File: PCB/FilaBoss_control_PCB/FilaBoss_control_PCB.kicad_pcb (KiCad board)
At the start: 2 copper layers, 1 part, among them U1 WEMOS_C3_mini

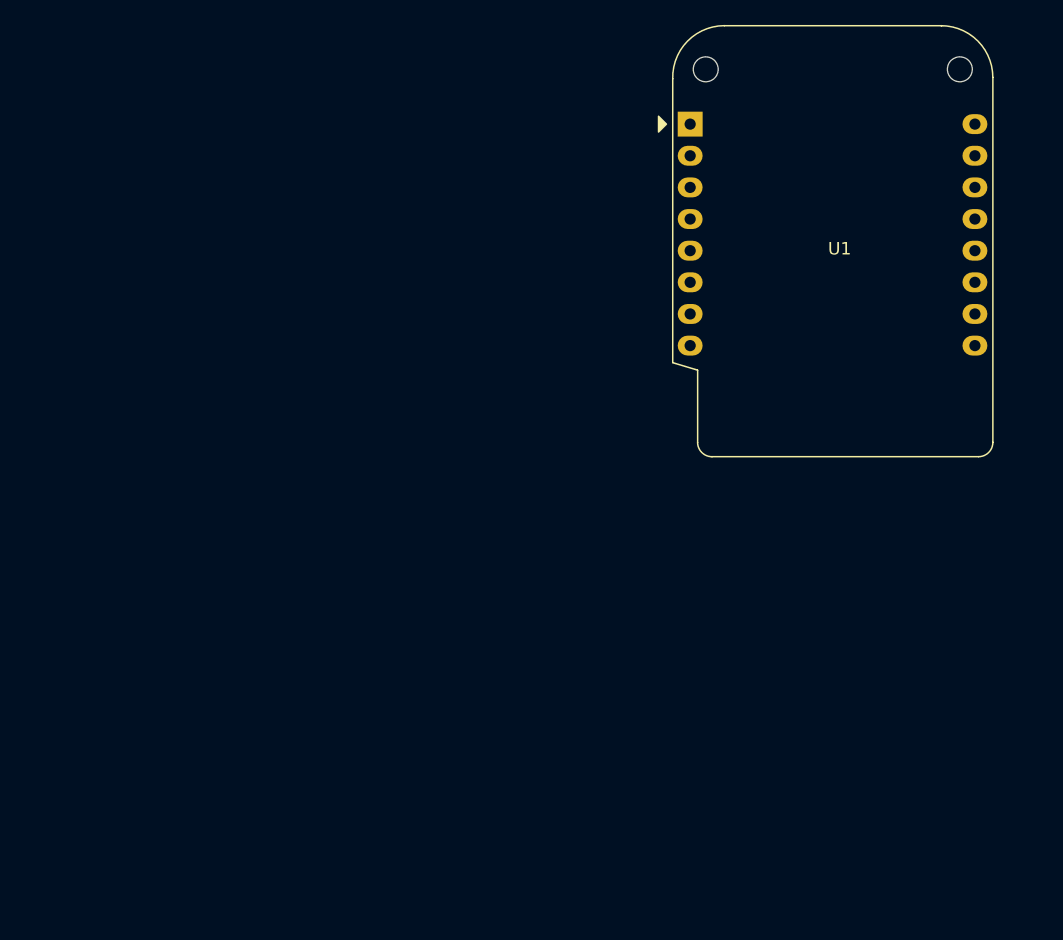
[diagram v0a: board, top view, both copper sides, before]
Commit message: pcb v1 ready
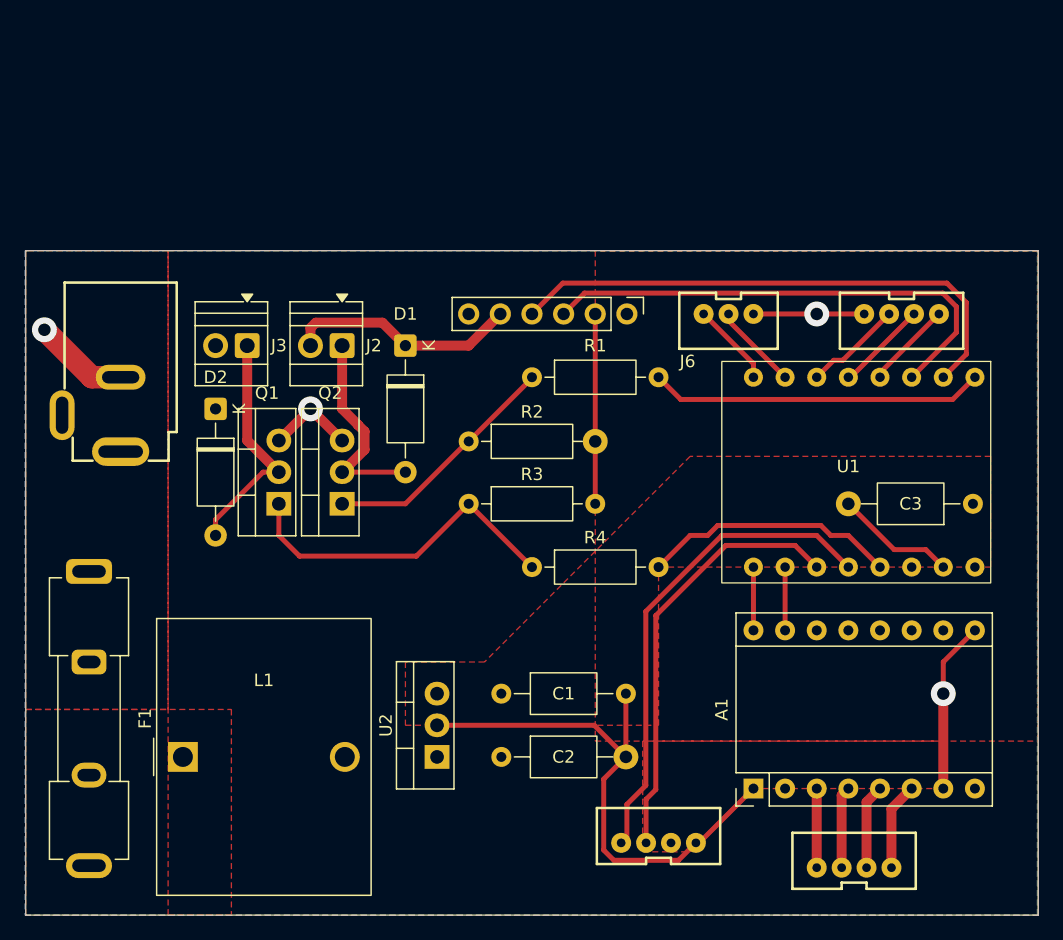
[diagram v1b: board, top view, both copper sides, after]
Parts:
- added A1: Pololu_Breakout_A4988, Module:Pololu_Breakout-16_15.2x20.3mm, F.Cu at (96.5, 129.5)
- added C1: C, Capacitor_THT:C_Axial_L5.1mm_D3.1mm_P10.00mm_Horizontal, F.Cu at (76.3, 121.9)
- added C2: C, Capacitor_THT:C_Axial_L5.1mm_D3.1mm_P10.00mm_Horizontal, F.Cu at (76.3, 127.0)
- added C3: C, Capacitor_THT:C_Axial_L5.1mm_D3.1mm_P10.00mm_Horizontal, F.Cu at (114.1, 106.7)
- added D1: D, Diode_THT:D_A-405_P10.16mm_Horizontal, F.Cu at (68.6, 94.0)
- added D2: D, Diode_THT:D_A-405_P10.16mm_Horizontal, F.Cu at (53.3, 99.1)
- added F1: Fuse, Fuse:Fuseholder_Clip-5x20mm_Keystone_3512P_Inline_P23.62x7.27mm_D1.02x2.41x1.02x1.57mm_Horizontal, F.Cu at (43.2, 112.1)
- added J1: Conn_01x04_Encoder, PCM_SparkFun-Connector:JST_1x04_P2.0mm_Vertical_PTH, F.Cu at (88.9, 133.3)
- added J2: Screw_Terminal_01x02, TerminalBlock:TerminalBlock_Xinya_XY308-2.54-2P_1x02_P2.54mm_Horizontal, F.Cu at (63.5, 94.0)
- added J3: Screw_Terminal_01x02, TerminalBlock:TerminalBlock_Xinya_XY308-2.54-2P_1x02_P2.54mm_Horizontal, F.Cu at (55.9, 94.0)
- added J5: Barrel_Jack_PTH_Slot, PCM_SparkFun-Connector:Barrel_Jack_PTH_Slot, F.Cu at (45.7, 96.5)
- added J6: PinHeader_01x06_P2.54mm_Vertical_THT_D1mm, PCM_fab:PinHeader_01x06_P2.54mm_Vertical_THT_D1mm, F.Cu at (86.4, 91.4)
- added J7: Conn_01x04, PCM_SparkFun-Connector:JST_1x04_P2.0mm_Vertical_PTH, F.Cu at (104.6, 135.3)
- added J8: JST_2mm_3, PCM_SparkFun-Connector:JST_1x03_P2.0mm_Vertical_PTH, F.Cu at (94.5, 92.0)
- added J9: Conn_01x04_Encoder, PCM_SparkFun-Connector:JST_1x04_P2.0mm_Vertical_PTH, F.Cu at (108.4, 92.0)
- added L1: L, Inductor_THT_Wurth:L_Wurth_WE-HCFT-2012_LeadDiameter1.2mm, F.Cu at (50.7, 127.0)
- added Q1: IRLZ44N, Package_TO_SOT_THT:TO-220-3_Vertical, F.Cu at (58.4, 106.7)
- added Q2: IRLZ44N, Package_TO_SOT_THT:TO-220-3_Vertical, F.Cu at (63.5, 106.7)
- added R1: 100R, Resistor_THT:R_Axial_DIN0207_L6.3mm_D2.5mm_P10.16mm_Horizontal, F.Cu at (78.7, 96.5)
- added R2: 10K, Resistor_THT:R_Axial_DIN0207_L6.3mm_D2.5mm_P10.16mm_Horizontal, F.Cu at (73.7, 101.7)
- added R3: 10K, Resistor_THT:R_Axial_DIN0207_L6.3mm_D2.5mm_P10.16mm_Horizontal, F.Cu at (73.7, 106.7)
- added R4: 100R, Resistor_THT:R_Axial_DIN0207_L6.3mm_D2.5mm_P10.16mm_Horizontal, F.Cu at (78.7, 111.8)
- added U2: LM78M05_TO220, Package_TO_SOT_THT:TO-220-3_Vertical, F.Cu at (71.1, 127.0)
- U1: value WEMOS_C3_mini -> ESP32_C3_super_mini; footprint RF_Module:WEMOS_C3_mini -> custom:ESP32-super-mini
- moved U1 31.8 mm to (106.7, 104.1), turned to -90 degrees
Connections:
- U1 pad 1: unconnected-(U1-EN-Pad1) -> Net-(A1-STEP)
- U1 pad 10: unconnected-(U1-GND-Pad10) -> Net-(J9-Pin_3)
- U1 pad 11: unconnected-(U1-D6-Pad11) -> +3.3V
- U1 pad 12: unconnected-(U1-D7-Pad12) -> GND
- U1 pad 13: unconnected-(U1-D8-Pad13) -> +5V
- U1 pad 2: unconnected-(U1-D3-Pad2) -> Net-(J1-Pin_2)
- U1 pad 3: unconnected-(U1-D2-Pad3) -> Net-(J1-Pin_1)
- U1 pad 4: unconnected-(U1-D1-Pad4) -> Net-(U1-D2/A2)
- U1 pad 5: unconnected-(U1-D0-Pad5) -> Net-(U1-D3/A3)
- U1 pad 6: unconnected-(U1-D4-Pad6) -> Net-(J6-Pin_4)
- U1 pad 7: unconnected-(U1-D5-Pad7) -> Net-(J6-Pin_3)
- U1 pad 8: unconnected-(U1-3V3-Pad8) -> Net-(J9-Pin_1)
- U1 pad 9: unconnected-(U1-VBus-Pad9) -> Net-(J9-Pin_2)
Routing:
- net GND: track 0.00 -> 106.7 mm, vias 0 -> 4
- net Net-(J6-Pin_4): track 0.00 -> 43.3 mm
- net Net-(J6-Pin_3): track 0.00 -> 39.8 mm
- net Net-(J1-Pin_1): track 0.00 -> 39.2 mm
- net Net-(J1-Pin_2): track 0.00 -> 34.5 mm
- net Net-(Q1-G): track 0.00 -> 27.4 mm
- net Net-(U1-D3/A3): track 0.00 -> 26.9 mm
- net Net-(U1-D2/A2): track 0.00 -> 20.5 mm
- net Net-(Q2-G): track 0.00 -> 19.6 mm
- net Net-(D2-A): track 0.00 -> 19.1 mm
- net Net-(D1-K): track 0.00 -> 18.6 mm
- net Net-(D1-A): track 0.00 -> 16.7 mm
- net Net-(J9-Pin_3): track 0.00 -> 7.91 mm
- net Net-(J9-Pin_2): track 0.00 -> 7.56 mm
- net Net-(J9-Pin_1): track 0.00 -> 7.04 mm
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- added copper zone on F.Cu, net +24V
- added copper zone on F.Cu, net +3.3V
- added copper zone on F.Cu, net +5V
- added copper zone on B.Cu, net GND
- added copper zone on F.Cu, net LINE
- added copper zone on F.Cu, net VDC
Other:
- board outline added: 81.3 x 53.3 mm
